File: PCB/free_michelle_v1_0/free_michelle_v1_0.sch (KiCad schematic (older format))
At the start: 12 parts

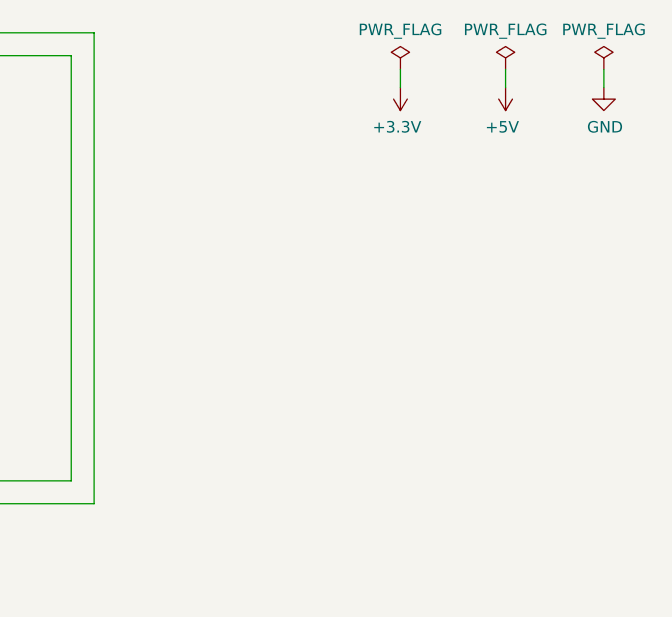
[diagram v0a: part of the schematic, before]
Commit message: Dodany L7805
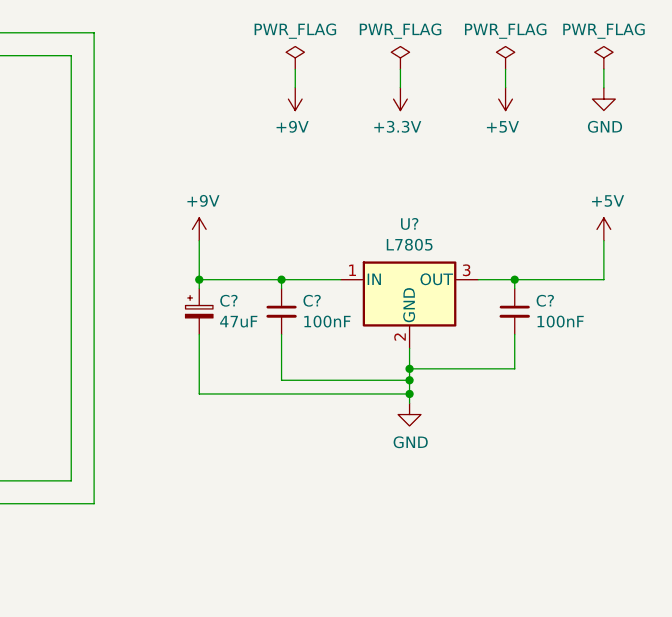
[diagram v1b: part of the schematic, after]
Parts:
- added C?: 47uF, symbol Device:CP_Small
- added C? (x2): 100nF, symbol Device:C_Small
- added U?: L7805, symbol Regulator_Linear:L7805
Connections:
- net +5V: now also C?.1, U?.3 (OUT)
- net GND: now also C?.2, C?.2, C?.2, U?.2 (GND)
- new net +9V: C?.1, C?.1, U?.1 (IN)
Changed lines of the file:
@@
 Wire Wire Line
 	2700 7330 2700 7300
+$Comp
+L power:PWR_FLAG #FLG?
+U 1 1 61DEC757
+P 12520 1060
+F 0 "#FLG?" H 12520 1135 50  0001 C CNN
+F 1 "PWR_FLAG" H 12520 1233 50  0000 C CNN
+F 2 "" H 12520 1060 50  0001 C CNN
+F 3 "~" H 12520 1060 50  0001 C CNN
+	1    12520 1060
+	1    0    0    -1
+$EndComp
+$Comp
+L power:+9V #PWR?
+U 1 1 61DEE2E8
+P 12520 1140
+F 0 "#PWR?" H 12520 990 50  0001 C CNN
+F 1 "+9V" H 12535 1313 50  0000 C CNN
+F 2 "" H 12520 1140 50  0001 C CNN
+F 3 "" H 12520 1140 50  0001 C CNN
+	1    12520 1140
+	-1   0    0    1
+$EndComp
+Wire Wire Line
+	12520 1140 12520 1060
+$Comp
+L Regulator_Linear:L7805 U?
+U 1 1 61DF26E8
+P 13020 1980
+F 0 "U?" H 13020 2222 50  0000 C CNN
+F 1 "L7805" H 13020 2131 50  0000 C CNN
+F 2 "" H 13045 1830 50  0001 L CIN
+F 3 "http://www.st.com/content/ccc/resource/technical/document/datasheet/41/4f/b3/b0/12/d4/47/88/CD00000444.pdf/files/CD00000444.pdf/jcr:content/translations/en.CD00000444.pdf" H 13020 1930 50  0001 C CNN
+	1    13020 1980
+	1    0    0    -1
+$EndComp
+$Comp
+L power:GND #PWR?
+U 1 1 61DF3DFA
+P 13020 2520
+F 0 "#PWR?" H 13020 2270 50  0001 C CNN
+F 1 "GND" H 13025 2347 50  0000 C CNN
+F 2 "" H 13020 2520 50  0001 C CNN
+F 3 "" H 13020 2520 50  0001 C CNN
+	1    13020 2520
+	1    0    0    -1
+$EndComp
+Wire Wire Line
+	13020 2520 13020 2480
+$Comp
+L power:+9V #PWR?
+U 1 1 61DF7AEA
+P 12100 1810
+F 0 "#PWR?" H 12100 1660 50  0001 C CNN
+F 1 "+9V" H 12115 1983 50  0000 C CNN
+F 2 "" H 12100 1810 50  0001 C CNN
+F 3 "" H 12100 1810 50  0001 C CNN
+	1    12100 1810
+	1    0    0    -1
+$EndComp
+Wire Wire Line
+	12100 1810 12100 1980
+$Comp
+L power:+5V #PWR?
+U 1 1 61DFBCEF
+P 13870 1810
+F 0 "#PWR?" H 13870 1660 50  0001 C CNN
+F 1 "+5V" H 13885 1983 50  0000 C CNN
+F 2 "" H 13870 1810 50  0001 C CNN
+F 3 "" H 13870 1810 50  0001 C CNN
+	1    13870 1810
+	1    0    0    -1
+$EndComp
+Wire Wire Line
+	13870 1810 13870 1980
+Wire Wire Line
+	13870 1980 13480 1980
+$Comp
+L Device:CP_Small C?
+U 1 1 61E00529
+P 12100 2120
+F 0 "C?" H 12188 2166 50  0000 L CNN
+F 1 "47uF" H 12188 2075 50  0000 L CNN
+F 2 "" H 12100 2120 50  0001 C CNN
+F 3 "~" H 12100 2120 50  0001 C CNN
+	1    12100 2120
+	1    0    0    -1
+$EndComp
+$Comp
+L Device:C_Small C?
+U 1 1 61E02529
+P 12460 2120
+F 0 "C?" H 12552 2166 50  0000 L CNN
+F 1 "100nF" H 12552 2075 50  0000 L CNN
+F 2 "" H 12460 2120 50  0001 C CNN
+F 3 "~" H 12460 2120 50  0001 C CNN
+	1    12460 2120
+	1    0    0    -1
+$EndComp
+Wire Wire Line
+	12100 1980 12460 1980
+Wire Wire Line
+	12100 2020 12100 1980
+Connection ~ 12100 1980
+Wire Wire Line
+	12460 2020 12460 1980
+Connection ~ 12460 1980
+Wire Wire Line
+	12460 1980 12720 1980
+Wire Wire Line
+	12100 2220 12100 2480
+Wire Wire Line
+	12100 2480 13020 2480
+Connection ~ 13020 2480
+Wire Wire Line
+	13020 2480 13020 2420
+Wire Wire Line
+	12460 2220 12460 2420
+Wire Wire Line
+	12460 2420 13020 2420
+Connection ~ 13020 2420
+Wire Wire Line
+	13020 2420 13020 2370
+$Comp
+L Device:C_Small C?
+U 1 1 61E310BD
+P 13480 2120
+F 0 "C?" H 13572 2166 50  0000 L CNN
+F 1 "100nF" H 13572 2075 50  0000 L CNN
+F 2 "" H 13480 2120 50  0001 C CNN
+F 3 "~" H 13480 2120 50  0001 C CNN
+	1    13480 2120
+	1    0    0    -1
+$EndComp
+Wire Wire Line
+	13480 2020 13480 1980
+Connection ~ 13480 1980
+Wire Wire Line
+	13480 1980 13320 1980
+Wire Wire Line
+	13480 2220 13480 2370
+Wire Wire Line
+	13480 2370 13020 2370
+Connection ~ 13020 2370
+Wire Wire Line
+	13020 2370 13020 2280
 $EndSCHEMATC
